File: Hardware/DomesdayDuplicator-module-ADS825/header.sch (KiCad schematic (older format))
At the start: 2 parts, among them J601 Back_connector, J602 Front_connector

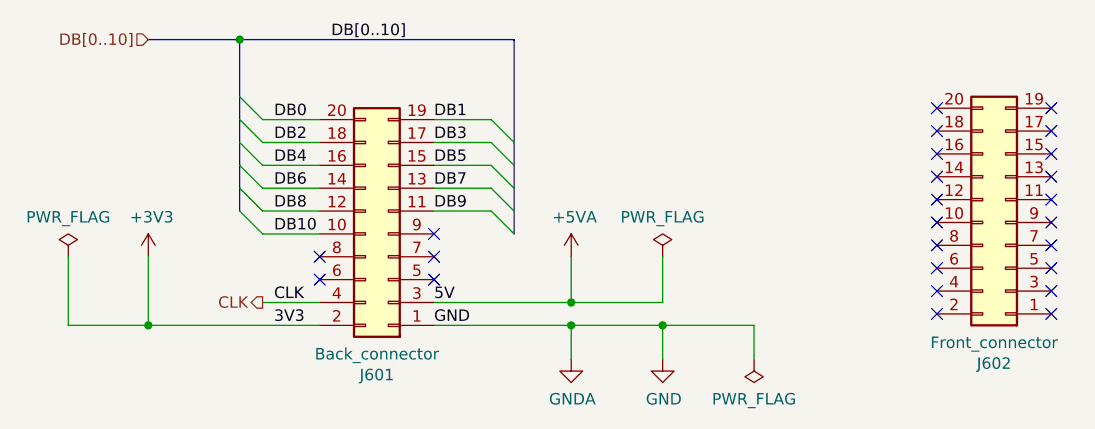
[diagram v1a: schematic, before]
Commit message: Work on the ADS825 module to determine the overall module dimensions and mounting
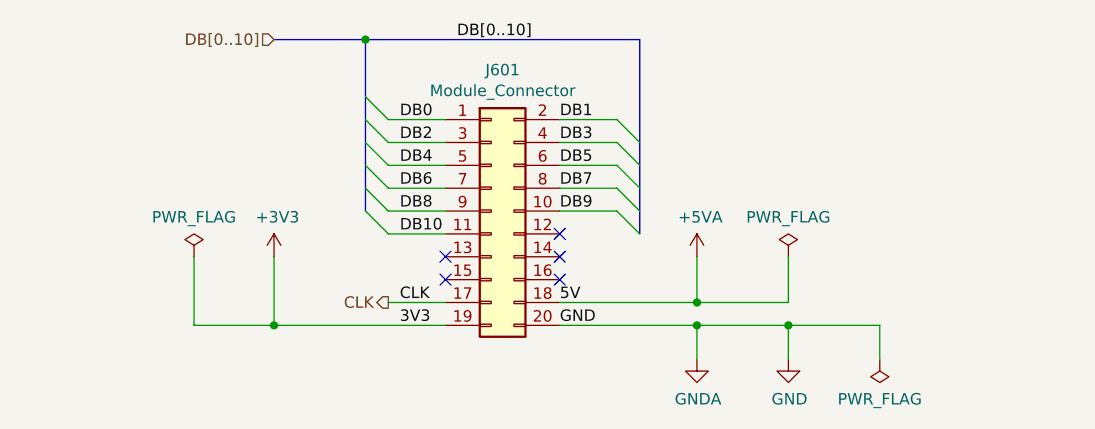
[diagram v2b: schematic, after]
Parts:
- removed J602: Front_connector, Connector_PinHeader_1.27mm:PinHeader_2x10_P1.27mm_Vertical_SMD, symbol Connector_Generic:Conn_02x10_Odd_Even
- J601: value Back_connector -> Module_Connector; footprint Connector_PinHeader_1.27mm:PinHeader_2x10_P1.27mm_Vertical_SMD -> Connector_PinSocket_2.54mm:PinSocket_2x10_P2.54mm_Vertical
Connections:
- net +3V3: now also J601.19 (Pin_19); no longer J601.2 (Pin_2)
- net +5VA: now also J601.18 (Pin_18); no longer J601.3 (Pin_3)
- net CLK: now also J601.17 (Pin_17); no longer J601.4 (Pin_4)
- net DB0: now also J601.1 (Pin_1); no longer J601.20 (Pin_20)
- net DB1: now also J601.2 (Pin_2); no longer J601.19 (Pin_19)
- net DB10: now also J601.11 (Pin_11); no longer J601.10 (Pin_10)
- net DB2: now also J601.3 (Pin_3); no longer J601.18 (Pin_18)
- net DB3: now also J601.4 (Pin_4); no longer J601.17 (Pin_17)
- net DB4: now also J601.5 (Pin_5); no longer J601.16 (Pin_16)
- net DB5: now also J601.6 (Pin_6); no longer J601.15 (Pin_15)
- net DB6: now also J601.7 (Pin_7); no longer J601.14 (Pin_14)
- net DB7: now also J601.8 (Pin_8); no longer J601.13 (Pin_13)
- net DB8: now also J601.9 (Pin_9); no longer J601.12 (Pin_12)
- net DB9: now also J601.10 (Pin_10); no longer J601.11 (Pin_11)
- net GND: now also J601.20 (Pin_20); no longer J601.1 (Pin_1)
- no-connect marks 25 -> 5
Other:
- moved on the sheet: J601
